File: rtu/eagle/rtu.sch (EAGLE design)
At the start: 109 parts

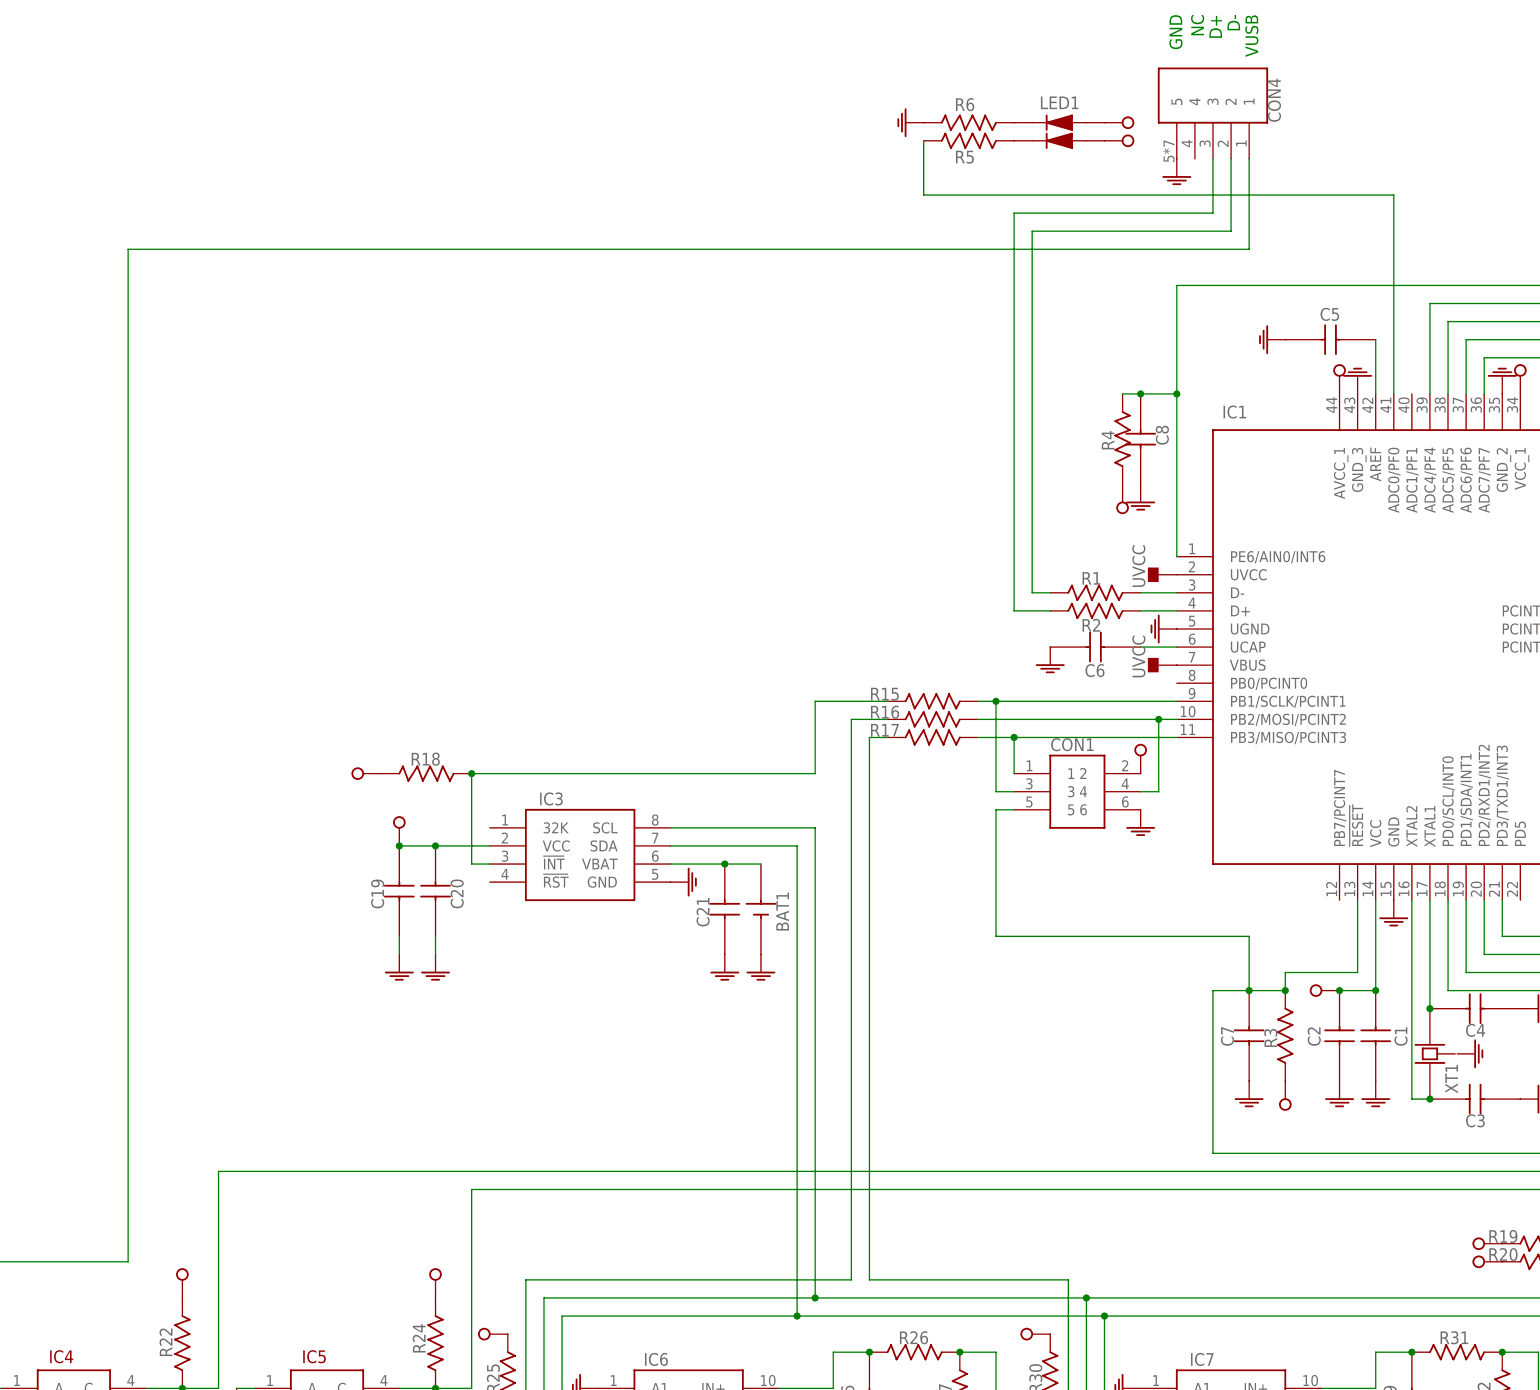
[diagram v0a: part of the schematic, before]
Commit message: do
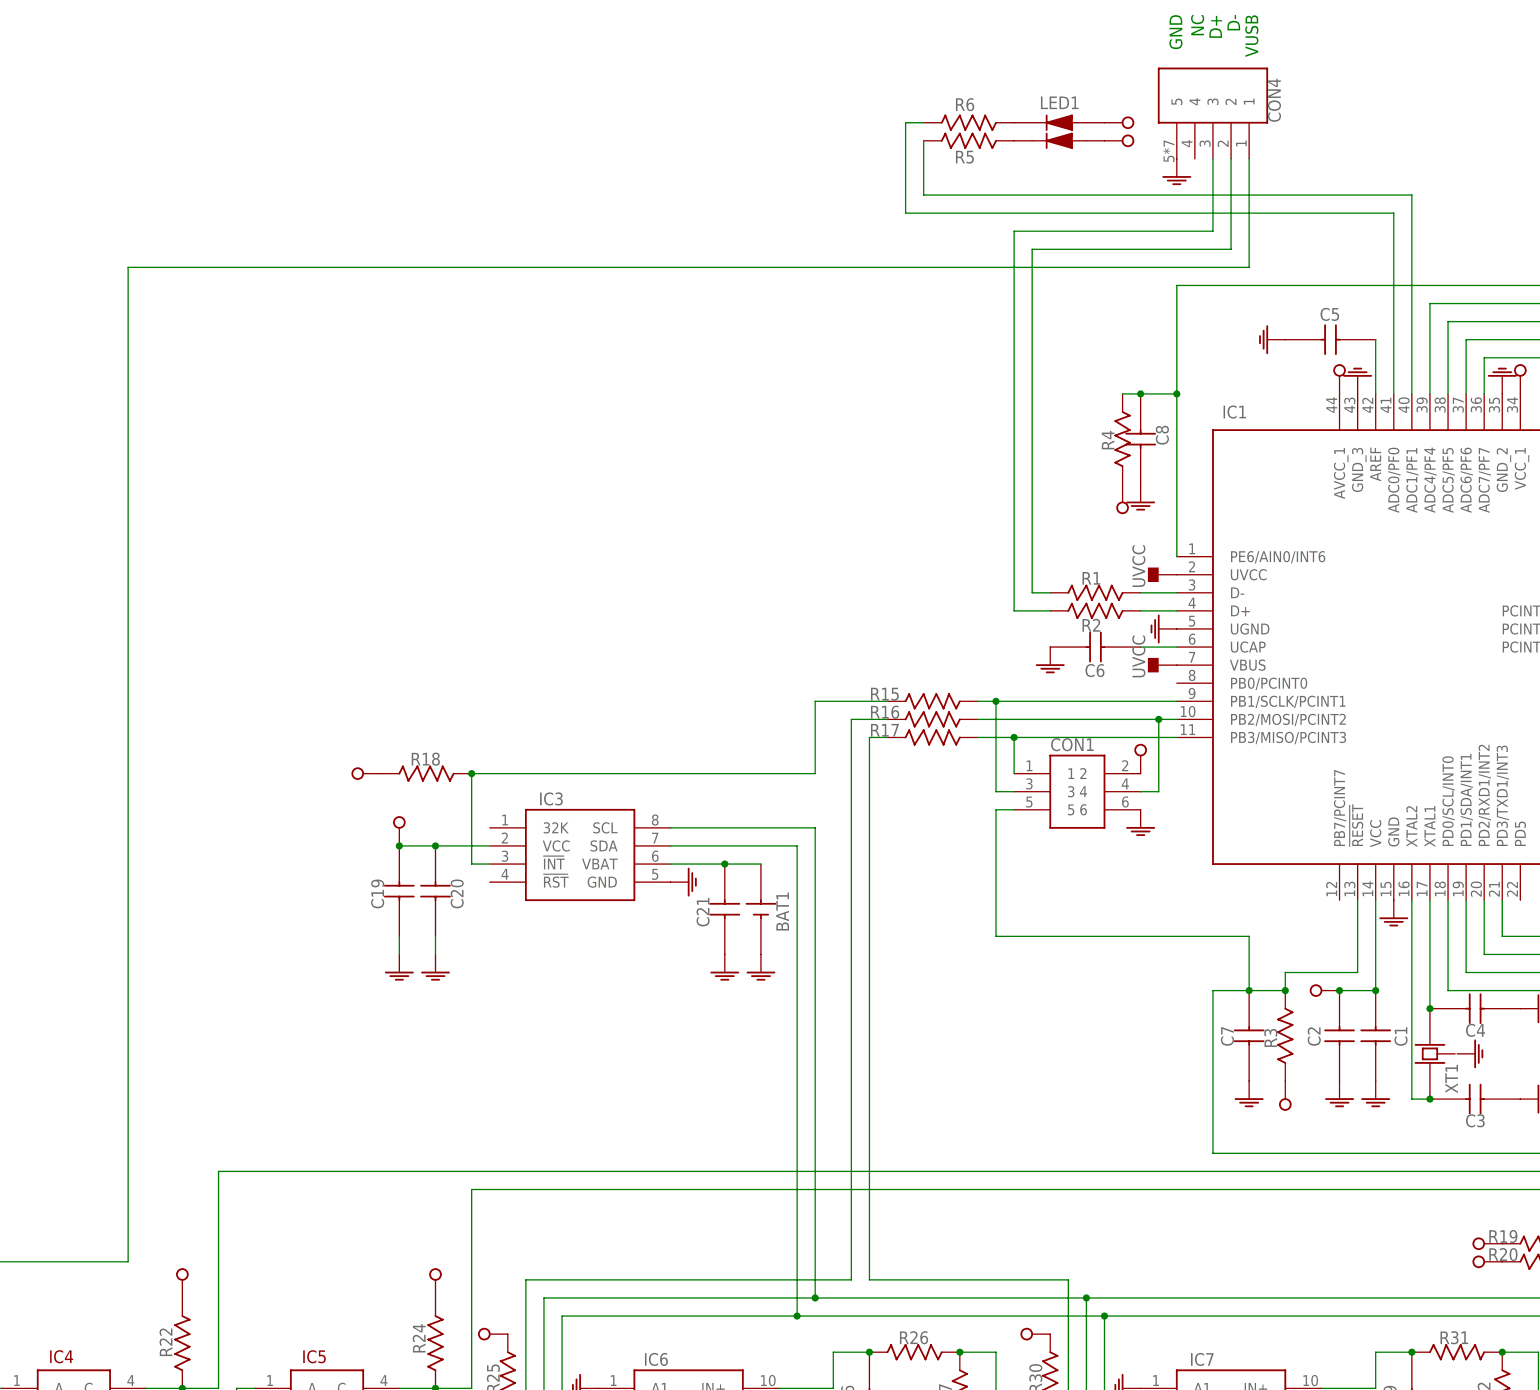
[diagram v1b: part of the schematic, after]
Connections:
- new net N$36: IC1.ADC0/PF0, R6.1
- net GND: no longer R6.1
- net N$1: now also IC1.ADC1/PF1; no longer IC1.ADC0/PF0
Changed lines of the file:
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@@
 <part name="R5" library="myparts" deviceset="RESISTOR-0603" device=""/>
 <part name="SUP7" library="myparts" deviceset="VCC" device=""/>
-<part name="GND25" library="myparts" deviceset="GND" device=""/>
 <part name="R38" library="myparts" deviceset="RESISTOR-0603" device=""/>
 <part name="R36" library="myparts" deviceset="RESISTOR-0603" device=""/>
@@
 <attribute name="VALUE" x="-41.275" y="73.025" size="1.778" layer="96" rot="R270"/>
 </instance>
-<instance part="GND25" gate="1" x="-73.66" y="73.66" smashed="yes" rot="R270">
-<attribute name="VALUE" x="-76.708" y="76.2" size="1.778" layer="96" rot="R270"/>
-</instance>
 <instance part="R38" gate="G$1" x="40.64" y="-109.22" smashed="yes">
 <attribute name="NAME" x="38.608" y="-108.204" size="1.778" layer="95" align="center-left"/>
@@
 <pinref part="C8" gate="G$1" pin="2"/>
 <pinref part="GND27" gate="1" pin="GND"/>
-</segment>
-<segment>
-<pinref part="R6" gate="G$1" pin="1"/>
-<pinref part="GND25" gate="1" pin="GND"/>
 </segment>
 <segment>
@@
 <pinref part="R1" gate="G$1" pin="1"/>
 <wire x1="-53.34" y1="7.62" x2="-55.88" y2="7.62" width="0.1524" layer="91"/>
-<wire x1="-55.88" y1="7.62" x2="-55.88" y2="58.42" width="0.1524" layer="91"/>
-<wire x1="-55.88" y1="58.42" x2="-27.94" y2="58.42" width="0.1524" layer="91"/>
-<wire x1="-27.94" y1="58.42" x2="-27.94" y2="68.58" width="0.1524" layer="91"/>
+<wire x1="-55.88" y1="7.62" x2="-55.88" y2="55.88" width="0.1524" layer="91"/>
+<wire x1="-55.88" y1="55.88" x2="-27.94" y2="55.88" width="0.1524" layer="91"/>
+<wire x1="-27.94" y1="55.88" x2="-27.94" y2="68.58" width="0.1524" layer="91"/>
 <pinref part="CON4" gate="G$1" pin="2"/>
 </segment>
@@
 <pinref part="R2" gate="G$1" pin="1"/>
 <wire x1="-53.34" y1="5.08" x2="-58.42" y2="5.08" width="0.1524" layer="91"/>
-<wire x1="-58.42" y1="5.08" x2="-58.42" y2="60.96" width="0.1524" layer="91"/>
-<wire x1="-58.42" y1="60.96" x2="-30.48" y2="60.96" width="0.1524" layer="91"/>
-<wire x1="-30.48" y1="60.96" x2="-30.48" y2="68.58" width="0.1524" layer="91"/>
+<wire x1="-58.42" y1="5.08" x2="-58.42" y2="58.42" width="0.1524" layer="91"/>
+<wire x1="-58.42" y1="58.42" x2="-30.48" y2="58.42" width="0.1524" layer="91"/>
+<wire x1="-30.48" y1="58.42" x2="-30.48" y2="68.58" width="0.1524" layer="91"/>
 <pinref part="CON4" gate="G$1" pin="3"/>
 </segment>
@@
 <pinref part="R5" gate="G$1" pin="1"/>
 <wire x1="-71.12" y1="63.5" x2="-71.12" y2="71.12" width="0.1524" layer="91"/>
-<pinref part="IC1" gate="G$1" pin="ADC0/PF0"/>
-<wire x1="-71.12" y1="63.5" x2="-5.08" y2="63.5" width="0.1524" layer="91"/>
-<wire x1="-5.08" y1="63.5" x2="-5.08" y2="35.56" width="0.1524" layer="91"/>
+<wire x1="-71.12" y1="63.5" x2="-2.54" y2="63.5" width="0.1524" layer="91"/>
+<pinref part="IC1" gate="G$1" pin="ADC1/PF1"/>
+<wire x1="-2.54" y1="63.5" x2="-2.54" y2="35.56" width="0.1524" layer="91"/>
 </segment>
 </net>
@@
 <wire x1="-327.66" y1="-106.68" x2="-327.66" y2="-86.36" width="0.1524" layer="91"/>
 <wire x1="-327.66" y1="-86.36" x2="-182.88" y2="-86.36" width="0.1524" layer="91"/>
-<wire x1="-182.88" y1="-86.36" x2="-182.88" y2="55.88" width="0.1524" layer="91"/>
-<wire x1="-25.4" y1="68.58" x2="-25.4" y2="55.88" width="0.1524" layer="91"/>
-<wire x1="-25.4" y1="55.88" x2="-182.88" y2="55.88" width="0.1524" layer="91"/>
+<wire x1="-182.88" y1="-86.36" x2="-182.88" y2="53.34" width="0.1524" layer="91"/>
+<wire x1="-25.4" y1="68.58" x2="-25.4" y2="53.34" width="0.1524" layer="91"/>
+<wire x1="-25.4" y1="53.34" x2="-182.88" y2="53.34" width="0.1524" layer="91"/>
 <pinref part="CON4" gate="G$1" pin="1"/>
 </segment>
@@
 </segment>
 </net>
+<net name="N$36" class="0">
+<segment>
+<pinref part="R6" gate="G$1" pin="1"/>
+<wire x1="-71.12" y1="73.66" x2="-73.66" y2="73.66" width="0.1524" layer="91"/>
+<wire x1="-73.66" y1="73.66" x2="-73.66" y2="60.96" width="0.1524" layer="91"/>
+<wire x1="-73.66" y1="60.96" x2="-5.08" y2="60.96" width="0.1524" layer="91"/>
+<pinref part="IC1" gate="G$1" pin="ADC0/PF0"/>
+<wire x1="-5.08" y1="60.96" x2="-5.08" y2="35.56" width="0.1524" layer="91"/>
+</segment>
+</net>
